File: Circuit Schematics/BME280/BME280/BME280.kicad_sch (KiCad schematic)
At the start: 8 parts, among them U1 BME280

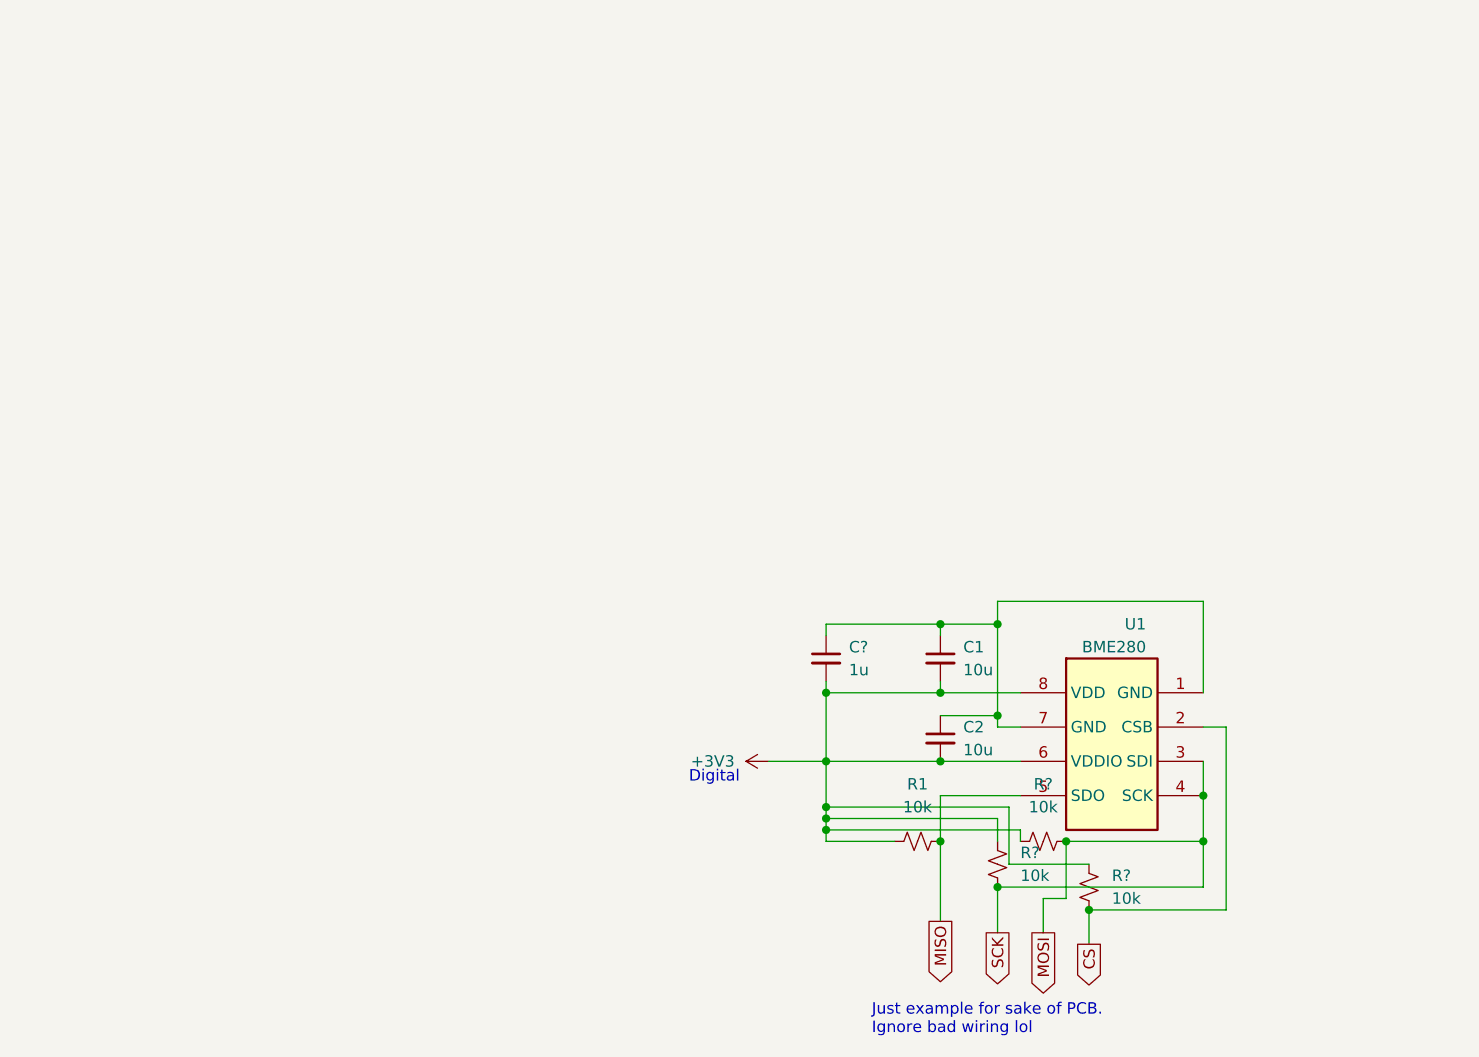
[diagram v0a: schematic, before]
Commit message: Whole boatload of changes
Latest.
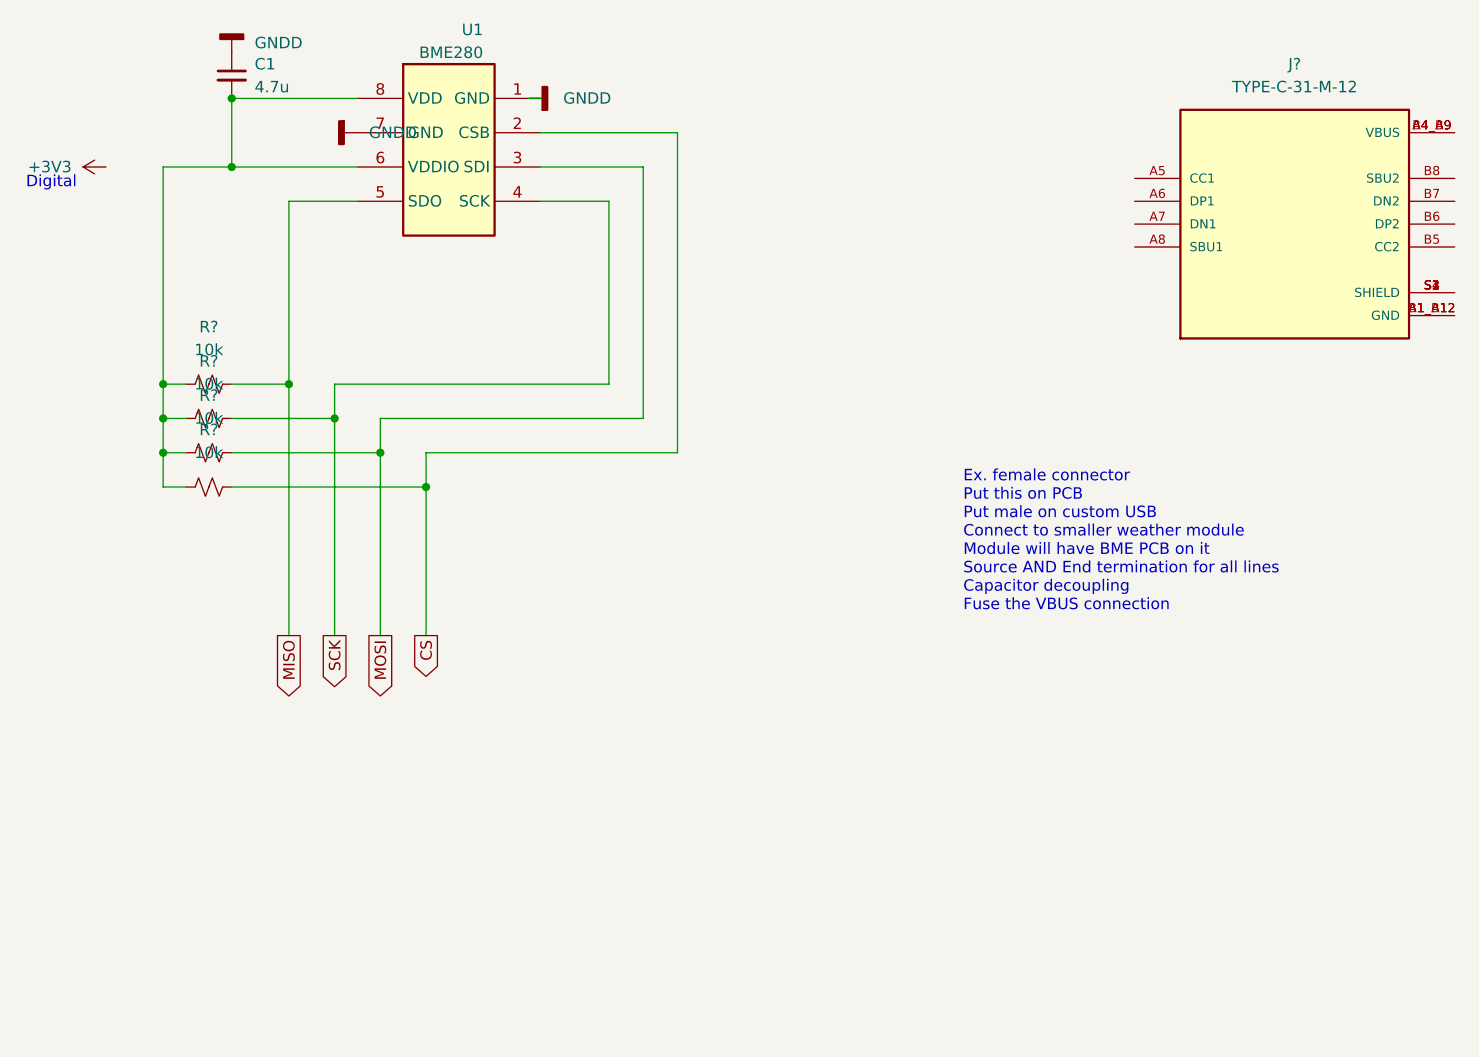
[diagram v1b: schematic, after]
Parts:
- removed C2: 10u, symbol Device:C_Small
- removed C?: 1u, symbol Device:C_Small
- removed R1, R? (x2): 10k, symbol Device:R_Small_US
- added J?: TYPE-C-31-M-12, HRO_TYPE-C-31-M-12, symbol TYPE-C-31-M-12:TYPE-C-31-M-12
- added R? (x3): 10k, symbol Device:R_Small_US
- C1: value 10u -> 4.7u
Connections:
- net +3V3: no longer C1.2, R?.2, U1.6 (VDDIO), U1.8 (VDD)
- net CS: now also R?.1
- net MISO: now also R?.1
- net MOSI: now also R?.1; no longer R?.1, U1.4 (SCK)
- net GNDD: now reaches C1.1, U1.1 (GND), U1.7 (GND)
- new net: C1.2, R?.2, R?.2, R?.2, R?.2, U1.6 (VDDIO), U1.8 (VDD)
- new net: J?.A1_B12 (GND), J?.B1_A12 (GND)
- new net: J?.A4_B9 (VBUS), J?.B4_A9 (VBUS)
- new net: J?.S1 (SHIELD), J?.S2 (SHIELD), J?.S3 (SHIELD), J?.S4 (SHIELD)
- new net SCK: R?.1, U1.4 (SCK)
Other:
- note added: "Ex. female connector Put this on PCB Put male on custom USB Connect to smaller weather module Module will have BME PCB on it Source AND End termination for all lines Capacitor decoupling Fuse the VBUS connection"
- note removed: "Just example for sake of PCB. Ignore bad wiring lol"
- moved on the sheet: C1, R?, U1
